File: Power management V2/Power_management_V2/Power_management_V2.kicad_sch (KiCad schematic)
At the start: 7 parts, among them J1 2165711003, U3 TPS3711DDCR

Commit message: Hoan thanh layout va BOM lisst
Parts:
- BAT1: Digikey WM11825-ND -> NC; JLCPCB Part # (none) -> NC; now left out of the parts list
- C34: JLCPCB Part # (none) -> C1591
- J1: Digikey (none) -> 900-2165711003-ND
- R15: Digikey (none) -> 311-2.00MHRCT-ND
- R16: Digikey (none) -> P51.1KHCT-ND
- U3: Digikey (none) -> 296-43278-1-ND
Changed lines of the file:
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@@
+			"AAAAAAAAAAAAAAAAAAAAAAAAAAAAAAAAAAAAAAAAAAAAAAAAAAAAAAAAAAAAAAAAAAAAAAAAAAAA"
+			"AAAAAAAAAAAAAAAAAAAAAAAAAAAAAAAAAAAAAAAAAAAAAAAAAAAAAAAAAAAAAAAAAAAAAAAAAAAA"
+			"AAAAAAAAAAAAAAAAAAAAAAAAAAAAAAAAAAAAAAAAAAAAAAAAAAAAAAAAAAAAAAAAAAAAAAAAAAAA"
+			"AAAAAAAAAAAAAAAAAAAAAAAAAAAAAAAAAAAAAAAAAAAAAAAAAAAAAAAAAAAAAAAAAAAAAAAAAAAA"
+			"AAAAAAAAAAAAAAAAAAAAAAAAAAAAAAAAAAAAAAAAAAAAAAAAAAAAAAAAAAAAAAAAAAAAAAAAAAAA"
+			"AAAAAAAAAAAAAAAAAAAAAAAAAAAAAAAAAAAAAAAAAAAAAAAAAAAAAAAAAAAAAAAAAAAAAAAAAAAA"
+			"AAAAAAAAAAAAAAAAAAAAAAAAAAAAAAAAAAAAAAAAAAAAAAAAAAAAAAAAAAAAAAAAAAAAAAAAAAAA"
+			"AAAAAAAAAAAAAAAAAAAAAAAAAAAAAAAAAAAAAAAAAAAAAAAAAAAAAAAAAAAAAAAAAAAAAAAAAAAA"
+			"AAAAAAAAAAAAAAAAAAAAAAAAAAAAAAAAAAAAAAAAAAAAAAAAAAAAAAAAAAAAAAAAAAAAAAAAAAAA"
+			"AAAAAAAAAAAAAAAAAAAAAAAAAAAAAAAAAAAAAAAAAAAAAAAAAAAAAAAAAAAAAAAAAAAAAAAAAAAA"
+			"AAAAAAAAAAAAAAAAAAAAAAAAAAAAAAAAAAAAAAAAAAAAAAAAAAAAAAAAAAAAAAAAAAAAAAAAAAAA"
+			"AAAAAAAAAAAAAAAAAAAAAAAAAAAAAAAAAAAAAAAAAAAAAAAAAAAAAAAAAAAAAAAAAAAAAAAAAAAA"
+			"AAAAAAAAAAAAAAAAAAAAAAAAAAAAAAAAAAAAAAAAAAAAAAAAAAAAAAAAAAAAAAAAAAAAAAAAAAAA"
+			"AAAAAAAAAAAAAAAAAAAAAAAAAAAAAAAAAAAAAAAAAAAAAAAAAAAAAAAAAAAAAAAAAAAAAAAAAAAA"
+			"AAAAAAAAAAAAAAAAAAAAAAAAAAAAAAAAAAAAAAAAAAAAAAAAAAAAAAAAAAAAAAAAAAAAAAAAAAAA"
+			"AAAAAAAAAAAAAAAAAAAAAAAAAAAAAAAAAAAAAAAAAAAAAAAAAAAAAAAAAAAAAAAAAAAAAAAAAAAA"
+			"AAAAAAAAAAAAAAAAAAAAAAAAAAAAAAAAAAAAAAAAAAAAAAAAAAAAAAAAAAAAAAAAAAAAAAAAAAAA"
+			"AAAAAAAAAAAAAAAAAAAAAAAAAAAAAAAAAAAAAAAAAAAAAAAAAAAAAAAAAAAAAAAAAAAAAAAAAAAA"
+			"AAAAAAAAAAAAAAAAAAAAAAAAAAAAAAAAAAAAAAAAAAAAAAAAAAAAAAAAAAAAAAAAAAAAAAAAAAAA"
+			"AAAAAAAAAAAAAAAAAAAAAAAAAAAAAAAAAAAAAAAAAAAAAAAAAAAAAAAAAAAAAAAAAAAAAAAAAAAA"
+			"AAAAAAAAAAAAAAAAAAAAAGUAbABsAGkAcABzAGkAcwAiAC8APgANAA0ACgA8AC8AaQBmAD4ADQAN"
+			"AAoAPABpAGYAIABzAGUAbABlAGMAdABlAGQAPQAiAGYAYQBsAHMAZQAiAD4ADQANAAoAPABlAGwA"
+			"ZQBtAGUAbgB0AA0ADQAKAHYAaQBzAGkAYgBsAGUAIAAgACAAIAAgACAAIAAgACAAIAA9ACAAIgBm"
+			"AGEAbABzAGUAIgANAA0ACgBlAG4AYQBiAGwAZQBkACAAIAAgACAAIAAgACAAIAAgACAAPQAgACIA"
+			"ZgBhAGwAcwBlACIADQANAAoALwA+AA0ADQAKADwALwBpAGYAPgANAA0ACgA8AC8AaQBmAD4ADQAN"
+			"AAoAPABpAGYAIABpAGQAPQAiAGEAdABvAG0AKABFAHgAcABhAG4AZABvAFQAZQB4AHQAQwBvAGwA"
+			"bABhAHAAcwBlAGQAKQAiAD4ADQANAAoAPABlAGwAZQBtAGUAbgB0AA0ADQAKAGYAbwBuAHQAIAAg"
+			"ACAAIAAgACAAIAAgACAAIAAgACAAIAAgACAAIAA9ACAAIgBnAHQAZgAoAFQAYQBzAGsARABpAGEA"
+			"bABvAGcAUwB0AHkAbABlACwAIAAxADIALAAgADAAKQAiAA0ADQAKAGYAbwByAGUAZwByAG8AdQBu"
+			"AGQAIAAgACAAIAAgACAAIAAgACAAIAA9ACAAIgBnAHQAYwAoAFQAYQBzAGsARABpAGEAbABvAGcA"
+			"UwB0AHkAbABlACwAIAAxADIALAAgADAALAAgADMAOAAwADMAKQAiAA0ADQAKAGMAbwBuAHQAZQBu"
+			"AHQAYQBsAGkAZwBuACAAIAAgACAAIAAgACAAIAA9ACAAIgB3AHIAYQBwAGwAZQBmAHQAIAB8ACAA"
+			"cABhAHQAaABlAGwAbABpAHAAcwBpAHMAIAB8ACAAdwBvAHIAZABlAGwAbABpAHAAcwBpAHMAIgAN"
+			"AA0ACgBwAGEAZABkAGkAbgBnACAAIAAgACAAIAAgACAAIAAgACAAIAAgACAAPQAgACIAdABoAGUA"
+			"bQBlAGEAYgBsAGUAKABnAHQAbQBhAHIAKABUAGEAcwBrAEQAaQBhAGwAbwBnACwAIAAxADIALAAg"
+			"ADAALAAgADMANgAwADIAKQAsACAAcgBlAGMAdAAoADAALAAyAHIAcAAsADAALAAwACkAKQAiAA0A"
+			"DQAKAHMAaABvAHIAdABjAHUAdAAgACAAIAAgACAAIAAgACAAIAAgACAAIAA9ACAAIgBhAHUAdABv"
+			"ACIADQANAAoALwA+AA0ADQAKADwAaQBmACAAawBlAHkAZgBvAGMAdQBzAGUAZAA9ACIAdAByAHUA"
+			"ZQAiAD4ADQANAAoAPABlAAAAAAAAAAAAAAAAAAAAAAAAAAAAAAAAAAAAAAAAAAAAAAAAAAAAAAAA"
+			"AAAAAAAAAAAAAAAAAAAAAAAAAAAAAAAAAAAAAAAAAAAAAAAAAAAAAAAAAAAAAAAAAAAAAAAAAAAA"
+			"AAAAAAAAAAAAAAAAAAAAAAAAAAAAAAAAAAAAAAAAAAAAAAAAAAAAAAAAAAAAAAAAAAAAAAAAAAAA"
+			"AAAAAAAAAAAAAAAAAAAAAAAAAAAAAAAAAAAAAAAAAAAAAAAAAAAAAAAAAAAAAAAAAAAAAAAAAAAA"
+			"AAAAAAAAAAAAAAAAAAAAAAAAAAAAAAAAAAAAAAAAAAAAAAAAAAAAAAAAAAAAAAAAAAAAAAAAAAAA"
+			"AAAAAAAAAAAAAAAAAAAAAAAAAAAAAAAAAAAAAAAAAAAAAAAAAAAAAAAAAAAAAAAAAAAAAAAAAAAA"
+			"AAAAAAAAAAAAAAAAAAAAAAAAAAAAAAAAAAAAAAAAAAAAAAAAAAAAAAAAAAAAAAAAAAAAAAAAAAAA"
+			"AAAAAAAAAAAAAAAAAAAAAAAAAAAAAAAAAAAAAAAAAAAAAAAAAAAAAAAAAAAAAAAAAAAAAAAAAAAA"
+			"AAAAAAAAAAAAAAAAAAAAAAAAAAAAAAAAAAAAAAAAAAAAAAAAAAAAAAAAAAAAAAAAAAAAAAAAAAAA"
+			"AAAAAAAAAAAAAAAAAAAAAAAAAAAAAAAAAAAAAAAAAAAAAAAAAAAAAAAAAAAAAAAAAAAAAAAAAAAA"
+			"AAAAAAAAAAAAAAAAAAAAAAAAAAAAAAAAAAAAAAAAAAAAAAAAAAAAAAAAAAAAAAAAAAAAAAAAAAAA"
+			"AAAAAAAAAAAAAAAAAAAAAAAAAAAAAAAAAAAAAAAAAAAAAAAAAAAAAAAAAAAAAAAAAAAAAAAAAAAA"
+			"AAAAAAAAAAAAAAAAAAAAAAAAAAAAAAAAAAAAAAAAAAAAAAAAAAAAAAAAAAAAAAAAAAAAAAAAAAAA"
+			"AAAAAAAAAAAAAAAAAAAAAAAAAAAAAAAAAAAAAAAAAAAAAAAAAAAAAAAAAAAAAAAAAAAAAAAAAAAA"
+			"AAAAAAAAAAAAAAAAAAAAAAAAAAAAAAAAAAAAAAAAAAAAAAAAAAAAAAAAAAAAAAAAAAAAAAAAAAAA"
+			"AAAAAAAAAAAAAAAAAAAAAAAAAAAAAAAAAAAAAAAAAAAAAAAAAAAAAAAAAAAAAAAAAAAAAAAAAAAA"
 			"AAAAAAAAAAAAAAAAAAAAAAAAAAAAAAAAAAAAAAAAAAAAAAAAAAAAAAAAAAAAAAAAAAAAAAAAAAAA"
 			"AAAAAAAAAAAAAAAAAAAAAAAAAAAAAAAAAAAAAAAAAAAAAAAAAAAAAAAAAAAAAAAAAAAAAAAAAAAA"
@@
 			)
 		)
-		(property "Digikey" ""
+		(property "Digikey" "P51.1KHCT-ND"
 			(at 61.595 99.695 0)
 			(effects
@@
 					(size 1.27 1.27)
 				)
+			)
+		)
+		(property "JLCPCB Part #" ""
+			(at 61.595 99.695 0)
+			(effects
+				(font
+					(size 1.27 1.27)
+				)
+				(hide yes)
 			)
 		)
@@
 			)
 		)
+		(property "JLCPCB Part #" ""
+			(at 112.395 78.74 0)
+			(effects
+				(font
+					(size 1.27 1.27)
+				)
+				(hide yes)
+			)
+		)
 		(pin "1"
 		)
@@
 					(size 1.27 1.27)
 				)
+			)
+		)
+		(property "JLCPCB Part #" "C1591"
+			(at 53.975 78.105 0)
+			(effects
+				(font
+					(size 1.27 1.27)
+				)
+				(hide yes)
 			)
 		)
@@
 		(unit 1)
 		(exclude_from_sim no)
-		(in_bom yes)
+		(in_bom no)
 		(on_board yes)
 		(dnp no)
@@
 			)
 		)
-		(property "Digikey" "WM11825-ND"
+		(property "Digikey" "NC"
 			(at 63.5 27.94 0)
 			(effects
@@
 					(size 1.27 1.27)
 				)
+			)
+		)
+		(property "JLCPCB Part #" "NC"
+			(at 63.5 27.94 0)
+			(effects
+				(font
+					(size 1.27 1.27)
+				)
+				(hide yes)
 			)
 		)
@@
 			)
 		)
+		(property "JLCPCB Part #" ""
+			(at 230.505 91.44 0)
+			(effects
+				(font
+					(size 1.27 1.27)
+				)
+				(hide yes)
+			)
+		)
+		(property "Digikey" "900-2165711003-ND"
+			(at 230.505 91.44 0)
+			(effects
+				(font
+					(size 1.27 1.27)
+				)
+				(hide yes)
+			)
+		)
 		(pin "2"
 		)
@@
 			)
 		)
+		(property "JLCPCB Part #" ""
+			(at 84.455 93.345 0)
+			(effects
+				(font
+					(size 1.27 1.27)
+				)
+				(hide yes)
+			)
+		)
+		(property "Digikey" "296-43278-1-ND"
+			(at 84.455 93.345 0)
+			(effects
+				(font
+					(size 1.27 1.27)
+				)
+				(hide yes)
+			)
+		)
 		(pin "6"
 		)
@@
 			)
 		)
-		(property "Digikey" ""
+		(property "Digikey" "311-2.00MHRCT-ND"
 			(at 61.595 90.805 0)
 			(effects
@@
 			)
 		)
+		(property "JLCPCB Part #" ""
+			(at 61.595 90.805 0)
+			(effects
+				(font
+					(size 1.27 1.27)
+				)
+				(hide yes)
+			)
+		)

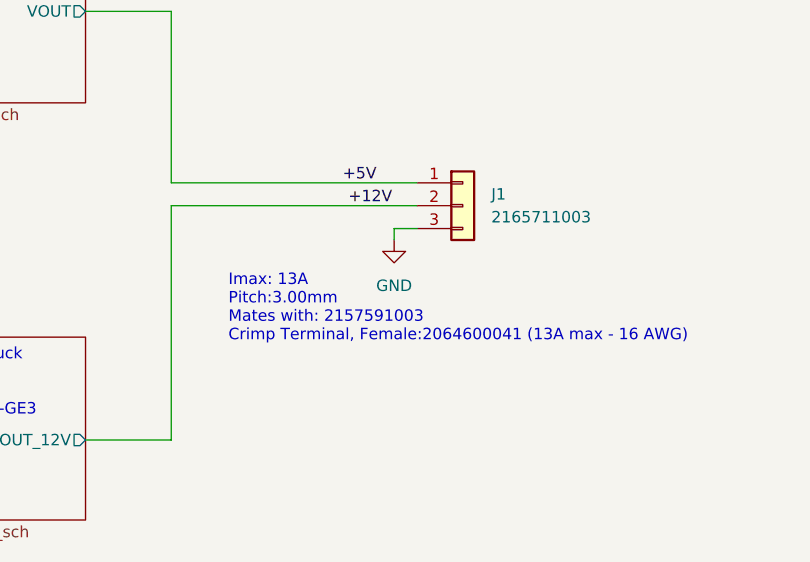
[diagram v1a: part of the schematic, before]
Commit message: Hoan thanh chinh sua 4/2
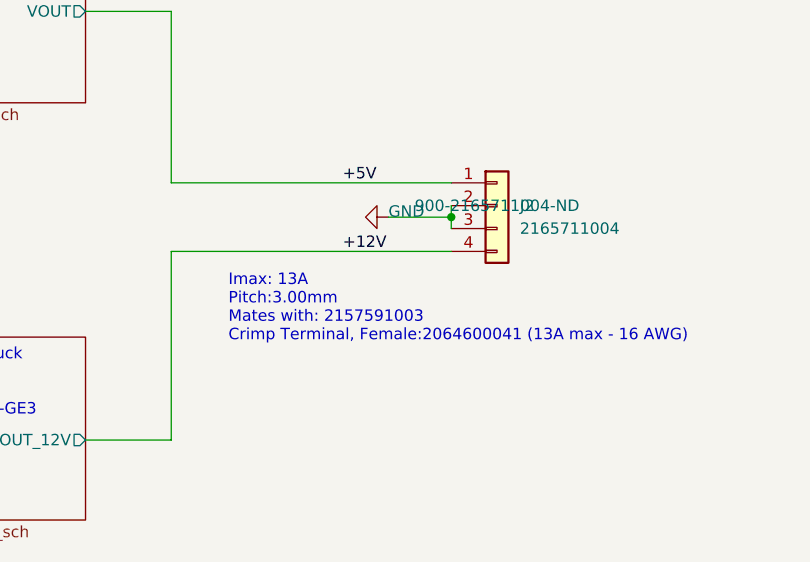
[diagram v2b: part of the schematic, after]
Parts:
- removed J1: 2165711003, Library:MOLEX_2165711003, symbol Connector_Generic:Conn_01x03
- added J2: 2165711004, Library:MOLEX_2165711004, symbol Connector_Generic:Conn_01x04
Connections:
- net +12V: now also J2.4 (Pin_4)
- net +5V: now also J2.1 (Pin_1)
- net GND: now also J2.2 (Pin_2), J2.3 (Pin_3)
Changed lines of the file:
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@@
+	)
+	(junction
+		(at 229.235 92.71)
+		(diameter 0)
+		(color 0 0 0 0)
 	)
 	(junction
@@
 	(wire
 		(pts
-			(xy 198.12 88.9) (xy 225.425 88.9)
+			(xy 222.25 92.71) (xy 229.235 92.71)
+		)
+		(stroke
+			(width 0)
+			(type default)
+		)
+	)
+	(wire
+		(pts
+			(xy 198.12 88.9) (xy 229.235 88.9)
+		)
+		(stroke
+			(width 0)
+			(type default)
+		)
+	)
+	(wire
+		(pts
+			(xy 229.235 92.71) (xy 229.235 93.98)
 		)
 		(stroke
@@
 	(wire
 		(pts
-			(xy 225.425 93.98) (xy 222.885 93.98)
-		)
-		(stroke
-			(width 0)
-			(type default)
-		)
-	)
-	(wire
-		(pts
 			(xy 57.15 27.94) (xy 57.15 26.67)
 		)
@@
 	(wire
 		(pts
-			(xy 198.12 91.44) (xy 225.425 91.44)
+			(xy 198.12 96.52) (xy 229.235 96.52)
 		)
 		(stroke
@@
 	(wire
 		(pts
-			(xy 198.12 117.475) (xy 198.12 91.44)
+			(xy 198.12 117.475) (xy 198.12 96.52)
 		)
 		(stroke
@@
 	(wire
 		(pts
+			(xy 229.235 91.44) (xy 229.235 92.71)
+		)
+		(stroke
+			(width 0)
+			(type default)
+		)
+	)
+	(wire
+		(pts
 			(xy 160.655 117.475) (xy 165.735 117.475)
 		)
@@
 		(pts
 			(xy 102.235 100.965) (xy 102.235 104.14)
-		)
-		(stroke
-			(width 0)
-			(type default)
-		)
-	)
-	(wire
-		(pts
-			(xy 222.885 93.98) (xy 222.885 95.25)
 		)
 		(stroke
@@
 			"AAAAAAAAAAAAAAAAAAAAAAAAAAAAAAAAAAAAAAAAAAAAAAAAAAAAAAAAAAAAAAAAAAAAAAAAAAAA"
 			"AAAAAAAAAAAAAAAAAAAAAAAAAAAAAAAAAAAAAAAAAAAAAAAAAAAAAAAAAAAAAAAAAAAAAAAAAAAA"
+			"AAAAAAAAAAAAAAAAAAAAAAAAAAAAAAAAAAAAAAAAAAAAAAAAAAAAAAAAAAAAAAAAAAAAAAAAAAAA"
+			"AAAAAAAAAAAAAAAAAAAAAAAAAAAAAAAAAAAAAAAAAAAAAAAAAAAAAAAAAAAAAAAAAAAAAAAAAAAA"
+			"AAAAAAAAAAAAAAAAAAAAAAAAAAAAAAAAAAAAAAAAAAAAAAAAAAAAAAAAAAAAAAAAAAAAAAAAAAAA"
+			"AAAAAAAAAAAAAAAAAAAAAAAAAAAAAAAAAAAAAAAAAAAAAAAAAAAAAAAAAAAAAAAAAAAAAAAAAAAA"
+			"AAAAAAAAAAAAAAAAAAAAAAAAAAAAAAAAAAAAAAAAAAAAAAAAAAAAAAAAAAAAAAAAAAAAAAAAAAAA"
+			"AAAAAAAAAAAAAAAAAAAAAAAAAAAAAAAAAAAAAAAAAAAAAAAAAAAAAAAAAAAAAAAAAAAAAAAAAAAA"
+			"AAAAAAAAAAAAAAAAAAAAAAAAAAAAAAAAAAAAAAAAAAAAAAAAAAAAAAAAAAAAAAAAAAAAAAAAAAAA"
+			"AAAAAAAAAAAAAAAAAAAAAAAAAAAAAAAAAAAAAAAAAAAAAAAAAAAAAAAAAAAAAAAAAAAAAAAAAAAA"
+			"AAAAAAAAAAAAAAAAAAAAAAAAAAAAAAAAAAAAAAAAAAAAAAAAAAAAAAAAAAAAAAAAAAAAAAAAAAAA"
+			"AAAAAAAAAAAAAAAAAAAAAAAAAAAAAAAAAAAAAAAAAAAAAAAAAAAAAAAAAAAAAAAAAAAAAAAAAAAA"
+			"AAAAAAAAAAAAAAAAAAAAAAAAAAAAAAAAAAAAAAAAAAAAAAAAAAAAAAAAAAAAAAAAAAAAAAAAAAAA"
+			"AAAAAAAAAAAAAAAAAAAAAAAAAAAAAAAAAAAAAAAAAAAAAAAAAAAAAAAAAAAAAAAAAAAAAAAAAAAA"
+			"AAAAAAAAAAAAAAAAAAAAAAAAAAAAAAAAAAAAAAAAAAAAAAAAAAAAAAAAAAAAAAAAAAAAAAAAAAAA"
+			"AAAAAAAAAAAAAAAAAAAAAAAAAAAAAAAAAAAAAAAAAAAAAAAAAAAAAAAAAAAAAAAAAAAAAAAAAAAA"
+			"AAAAAAAAAAAAAAAAAAAAAAAAAAAAAAAAAAAAAAAAAAAAAAAAAAAAAAAAAAAAAAAAAAAAAAAAAAAA"
+			"AAAAAAAAAAAAAAAAAAAAAAAAAAAAAAAAAAAAAAAAAAAAAAAAAAAAAAAAAAAAAAAAAAAAAAAAAAAA"
+			"AAAAAAAAAAAAAAAAAAAAAAAAAAAAAAAAAAAAAAAAAAAAAAAAAAAAAAAAAAAAAAAAAAAAAAAAAAAA"
+			"AAAAAAAAAAAAAAAAAAAAAAAAAAAAAAAAAAAAAAAAAAAAAAAAAAAAAAAAAAAAAAAAAAAAAAAAAAAA"
+			"AAAAAAAAAAAAAAAAAAAAAAAAAAAAAAAAAAAAAAAAAAAAAAAAAAAAAAAAAAAAAAAAAAAAAAAAAAAA"
+			"AAAAAAAAAAAAAAAAAAAAAAAAAAAAAAAAAAAAAAAAAAAAAAAAAAAAAAAAAAAAAAAAAAAAAAAAAAAA"
+			"AAAAAAAAAAAAAAAAAAAAAAAAAAAAAAAAAAAAAAAAAAAAAAAAAAAAAAAAAAAAAAAAAAAAAAAAAAAA"
+			"AAAAAAAAAAAAAAAAAAAAAAAAAAAAAAAAAAAAAAAAAAAAAAAAAAAAAAAAAAAAAAAAAAAAAAAAAAAA"
+			"AAAAAAAAAAAAAAAAAAAAAAAAAAAAAAAAAAAAAAAAAAAAAAAAAAAAAAAAAAAAAAAAAAAAAAAAAAAA"
+			"AAAAAAAAAAAAAAAAAAAAAAAAAAAAAAAAAAAAAAAAAAAAAAAAAAAAAAAAAAAAAAAAAAAAAAAAAAAA"
+			"AAAAAAAAAAAAAAAAAAAAAAAAAAAAAAAAAAAAAAAAAAAAAAAAAAAAAAAAAAAAAAAAAAAAAAAAAAAA"
+			"AAAAAAAAAAAAAAAAAAAAAAAAAAAAAAAAAAAAAAAAAAAAAAAAAAAAAAAAAAAAAAAAAAAAAAAAAAAA"
+			"AAAAAAAAAAAAAAAAAAAAAAAAAAAAAAAAAAAAAAAAAAAAAAAAAAAAAAAAAAAAAAAAAAAAAAAAAAAA"
+			"AAAAAAAAAAAAAAAAAAAAAAAAAAAAAAAAAAAAAAAAAAAAAAAAAAAAAAAAAAAAAAAAAAAAAAAAAAAA"
+			"AAAAAAAAAAAAAAAAAAAAAAAAAAAAAAAAAAAAAAAAAAAAAAAAAAAAAAAAAAAAAAAAAAAAAAAAAAAA"
+			"AAAAAAAAAAAAAAAAAAAAAAAAAAAAAAAAAAAAAAAAAAAAAAAAAAAAAAAAAAAAAAAAAAAAAAAAAAAA"
+			"AAAAAAAAAAAAAAAAAAAAAAAAAAAAAAAAAAAAAAAAAAAAAAAAAAAAAAAAAAAAAAAAAAAAAAAAAAAA"
+			"AAAAAAAAAAAAAAAAAAAAAAAAAAAAAAAAAAAAAAAAAAAAAAAAAAAAAAAAAAAAAAAAAAAAAAAAAAAA"
+			"AAAAAAAAAAAAAAAAAAAAAAAAAAAAAAAAAAAAAAAAAAAAAAAAAAAAAAAAAAAAAAAAAAAAAAAAAAAA"
+			"AAAAAAAAAAAAAAAAAAAAAAAAAAAAAAAAAAAAAAAAAAAAAAAAAAAAAAAAAAAAAAAAAAAAAAAAAAAA"
+			"AAAAAAAAAAAAAAAAAAAAAAAAAAAAAAAAAAAAAAAAAAAAAAAAAAAAAAAAAAAAAAAAAAAAAAAAAAAA"
+			"AAAAAAAAAAAAAAAAAAAAAAAAAAAAAAAAAAAAAAAAAAAAAAAAAAAAAAAAAAAAAAAAAAAAAAAAAAAA"
 			"AAAAAAAAAAAAAAAAAAAAAA=="
 		)
 	)
 	(label "+12V"
-		(at 217.805 91.44 0)
+		(at 217.17 96.52 0)
 		(effects
 			(font
@@
 	)
 	(symbol
-		(lib_id "Connector_Generic:Conn_01x03")
-		(at 230.505 91.44 0)
+		(lib_id "Connector_Generic:Conn_01x04")
+		(at 234.315 91.44 0)
 		(unit 1)
 		(exclude_from_sim no)
@@
 		(dnp no)
 		(fields_autoplaced yes)
-		(property "Reference" "J1"
-			(at 233.68 90.1699 0)
+		(property "Reference" "J2"
+			(at 236.855 91.4399 0)
 			(effects
 				(font
@@
 			)
 		)
-		(property "Value" "2165711003"
-			(at 233.68 92.7099 0)
+		(property "Value" "2165711004"
+			(at 236.855 93.9799 0)
 			(effects
 				(font
@@
 			)
 		)
-		(property "Footprint" "Library:MOLEX_2165711003"
-			(at 230.505 91.44 0)
+		(property "Footprint" "Library:MOLEX_2165711004"
+			(at 234.315 91.44 0)
 			(effects
 				(font
@@
 		)
 		(property "Datasheet" "~"
-			(at 230.505 91.44 0)
-			(effects
-				(font
-					(size 1.27 1.27)
-				)
-				(hide yes)
-			)
-		)
-		(property "Description" "Generic connector, single row, 01x03, script generated (kicad-library-utils/schlib/autogen/connector/)"
-			(at 230.505 91.44 0)
-			(effects
-				(font
-					(size 1.27 1.27)
-				)
-				(hide yes)
-			)
-		)
-		(property "Sim.Device" ""
-			(at 230.505 91.44 0)
-			(effects
-				(font
-					(size 1.27 1.27)
-				)
-			)
-		)
-		(property "Sim.Params" ""
-			(at 230.505 91.44 0)
-			(effects
-				(font
-					(size 1.27 1.27)
-				)
-			)
-		)
-		(property "Sim.Pins" ""
-			(at 230.505 91.44 0)
-			(effects
-				(font
-					(size 1.27 1.27)
-				)
-			)
-		)
-		(property "JLCPCB Part #" ""
-			(at 230.505 91.44 0)
-			(effects
-				(font
-					(size 1.27 1.27)
-				)
-				(hide yes)
-			)
-		)
-		(property "Digikey" "900-2165711003-ND"
-			(at 230.505 91.44 0)
-			(effects
-				(font
-					(size 1.27 1.27)
-				)
-				(hide yes)
-			)
+			(at 234.315 91.44 0)
+			(effects
+				(font
+					(size 1.27 1.27)
+				)
+				(hide yes)
+			)
+		)
+		(property "Description" "Generic connector, single row, 01x04, script generated (kicad-library-utils/schlib/autogen/connector/)"
+			(at 234.315 91.44 0)
+			(effects
+				(font
+					(size 1.27 1.27)
+				)
+				(hide yes)
+			)
+		)
+		(property "DIGIKEY" "900-2165711004-ND"
+			(at 234.315 91.44 0)
+			(effects
+				(font
+					(size 1.27 1.27)
+				)
+				(hide yes)
+			)
+		)
+		(property "Digikey" "900-2165711004-ND"
+			(at 234.315 91.44 0)
+			(effects
+				(font
+					(size 1.27 1.27)
+				)
+			)
+		)
+		(pin "1"
 		)
 		(pin "2"
@@
 		(pin "3"
 		)
-		(pin "1"
+		(pin "4"
 		)
 		(instances
 			(project ""
 				(path "/632966f8-0e72-49d8-ae31-468f807051b0"
-					(reference "J1")
+					(reference "J2")
 					(unit 1)
 				)
@@
 	(symbol
 		(lib_id "power:GND")
-		(at 222.885 95.25 0)
+		(at 222.25 92.71 270)
 		(unit 1)
 		(exclude_from_sim no)
@@
 		(on_board yes)
 		(dnp no)
-		(fields_autoplaced yes)
 		(property "Reference" "#PWR05"
-			(at 222.885 101.6 0)
+			(at 215.9 92.71 0)
 			(effects
 				(font
@@
 		)
 		(property "Value" "GND"
-			(at 222.885 100.33 0)
-			(effects
-				(font
-					(size 1.27 1.27)
-				)
+			(at 222.25 92.075 90)
+			(effects
+				(font
+					(size 1.27 1.27)
+				)
+				(justify left)
 			)
 		)
 		(property "Footprint" ""
-			(at 222.885 95.25 0)
+			(at 222.25 92.71 0)
 			(effects
 				(font
@@
 		)
 		(property "Datasheet" ""
-			(at 222.885 95.25 0)
+			(at 222.25 92.71 0)
 			(effects
 				(font
@@
 		)
 		(property "Description" ""
-			(at 222.885 95.25 0)
-			(effects
-				(font
+			(at 222.25 92.71 0)
+			(effects
+				(font
